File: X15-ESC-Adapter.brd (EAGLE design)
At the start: 101.6 x 41.1 mm, 10 parts, among them J1 IPBT-103-H1-T-S, J2 IPBT-103-H1-T-S, J3 IPBT-103-H1-T-S, J4 IPBT-103-H1-T-S

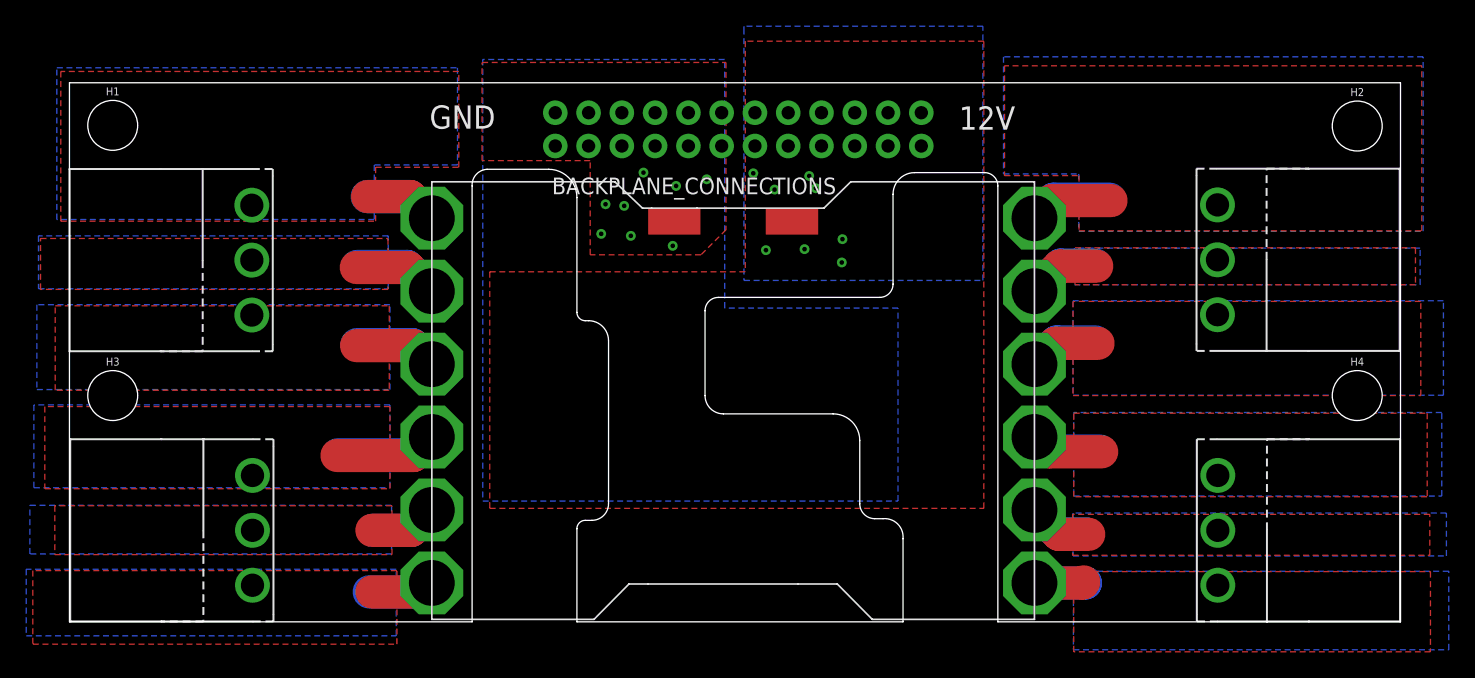
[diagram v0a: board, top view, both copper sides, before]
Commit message: 4th Final Version
Fixed errors
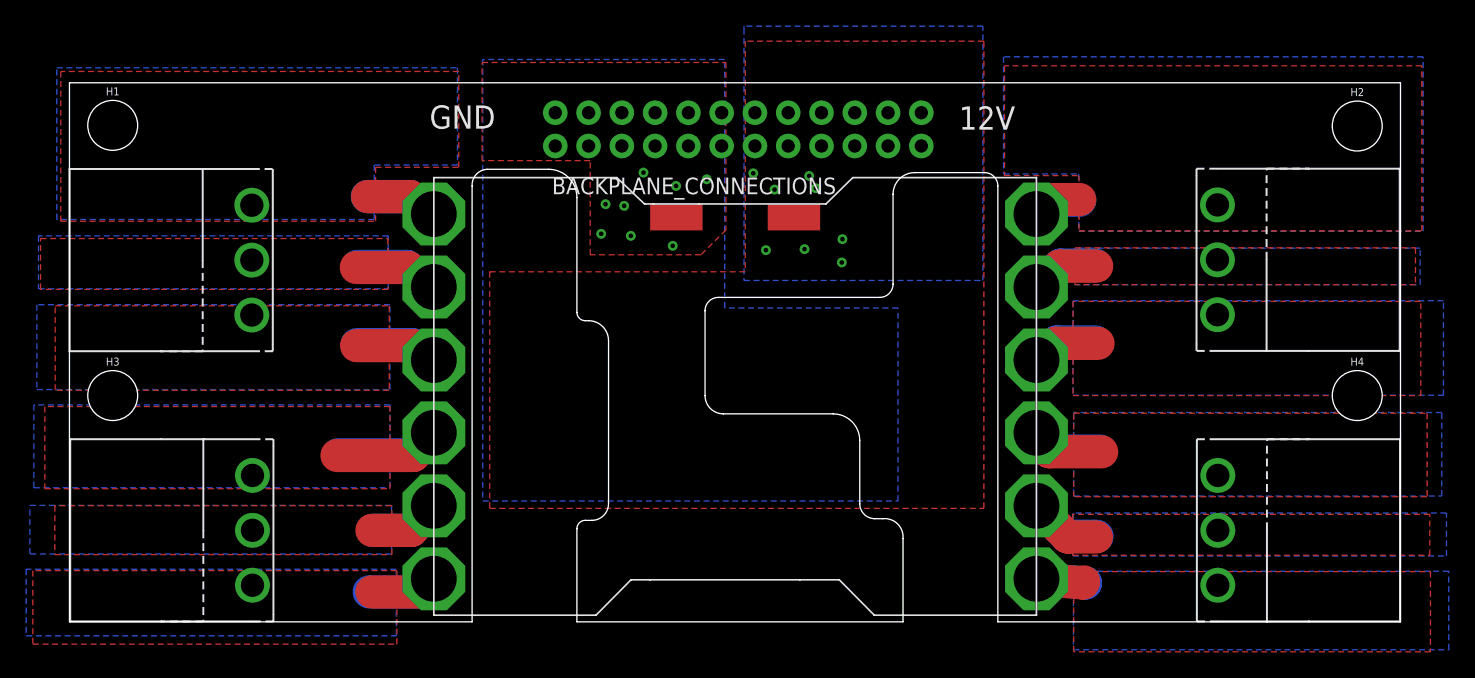
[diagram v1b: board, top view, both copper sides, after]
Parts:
- moved LUMENIER_ESC 0.35 mm to (27.8, 0.51)
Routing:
- net ESC3_B: track 12.7 -> 7.41 mm
- net ESC4_Y: track 9.55 -> 11.1 mm
- net ESC2_R: track 9.91 -> 10.6 mm
- net ESC2_B: track 15.5 -> 16.2 mm
- net ESC2_Y: track 10.4 -> 11.1 mm
- net ESC3_Y: track 11.0 -> 10.4 mm
- net ESC3_R: track 10.9 -> 10.2 mm
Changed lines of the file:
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@@
 <param name="mdViaViaSameLayer" value="6mil"/>
 <param name="mnLayersViaInSmd" value="2"/>
-<param name="mdCopperDimension" value="40mil"/>
+<param name="mdCopperDimension" value="15mil"/>
 <param name="mdDrill" value="6mil"/>
 <param name="mdSmdStop" value="0mil"/>
@@
 <element name="J3" library="X15-ESC-Adapter" package="IPBT-103-H1-T-S" value="IPBT-103-H1-T-S" x="87.63" y="27.6352" smashed="yes" rot="R270"/>
 <element name="J4" library="X15-ESC-Adapter" package="IPBT-103-H1-T-S" value="IPBT-103-H1-T-S" x="87.6554" y="6.985" smashed="yes" rot="R270"/>
-<element name="LUMENIER_ESC" library="X15-ESC-Adapter" package="LUMENIER" package3d_urn="urn:adsk.eagle:package:24294694/3" value="LUMENIER" x="27.66" y="0.1892" smashed="yes"/>
+<element name="LUMENIER_ESC" library="X15-ESC-Adapter" package="LUMENIER" package3d_urn="urn:adsk.eagle:package:24294694/3" value="LUMENIER" x="27.813" y="0.508" smashed="yes"/>
 </elements>
 <signals>
@@
 <vertex x="104.8766" y="24.511"/>
 </polygon>
-<wire x1="73.66" y1="19.6692" x2="75.2506" y2="21.2598" width="2.54" layer="1"/>
+<wire x1="73.813" y1="19.988" x2="75.2506" y2="21.2598" width="2.54" layer="1"/>
 <wire x1="75.2506" y1="21.2598" x2="78.5114" y2="21.2598" width="2.54" layer="1"/>
-<wire x1="73.66" y1="19.6692" x2="75.3522" y2="21.3614" width="2.54" layer="16"/>
+<wire x1="73.813" y1="19.988" x2="75.3522" y2="21.3614" width="2.54" layer="16"/>
 <wire x1="75.3522" y1="21.3614" x2="78.3082" y2="21.3614" width="2.54" layer="16"/>
 </signal>
@@
 <vertex x="103.0986" y="28.5242"/>
 </polygon>
-<wire x1="73.66" y1="25.2392" x2="75.5734" y2="27.1526" width="2.54" layer="1"/>
+<wire x1="73.813" y1="25.558" x2="75.5734" y2="27.1526" width="2.54" layer="1"/>
 <wire x1="75.5734" y1="27.1526" x2="78.4098" y2="27.1526" width="2.54" layer="1"/>
-<wire x1="73.66" y1="25.2392" x2="75.6496" y2="27.2288" width="2.54" layer="16"/>
+<wire x1="73.813" y1="25.558" x2="75.6496" y2="27.2288" width="2.54" layer="16"/>
 <wire x1="75.6496" y1="27.2288" x2="78.3082" y2="27.2288" width="2.54" layer="16"/>
 </signal>
@@
 <vertex x="103.3272" y="43.1292"/>
 </polygon>
-<wire x1="73.66" y1="30.8092" x2="75.0072" y2="32.1564" width="2.54" layer="1"/>
-<wire x1="75.0072" y1="32.1564" x2="79.502" y2="32.1564" width="2.54" layer="1"/>
-<wire x1="73.66" y1="30.8092" x2="75.1088" y2="32.258" width="2.54" layer="16"/>
-<wire x1="75.1088" y1="32.258" x2="79.4004" y2="32.258" width="2.54" layer="16"/>
+<wire x1="73.813" y1="31.128" x2="75.0834" y2="32.2326" width="2.54" layer="1"/>
+<wire x1="75.0834" y1="32.2326" x2="77.1144" y2="32.2326" width="2.54" layer="1"/>
+<wire x1="73.813" y1="31.128" x2="75.0326" y2="32.1818" width="2.54" layer="16"/>
+<wire x1="75.0326" y1="32.1818" x2="77.1144" y2="32.1818" width="2.54" layer="16"/>
 </signal>
 <signal name="ESC4_R">
@@
 <vertex x="105.283" y="3.8608"/>
 </polygon>
-<wire x1="73.66" y1="2.9692" x2="77.3404" y2="2.9692" width="2.54" layer="1"/>
+<wire x1="73.813" y1="3.288" x2="77.3404" y2="2.9692" width="2.54" layer="1"/>
 <wire x1="77.3404" y1="2.9692" x2="77.4192" y2="3.048" width="2.54" layer="1"/>
-<wire x1="73.66" y1="2.9692" x2="77.5436" y2="2.9692" width="2.54" layer="16"/>
+<wire x1="73.813" y1="3.288" x2="77.5436" y2="2.9692" width="2.54" layer="16"/>
 <wire x1="77.5436" y1="2.9692" x2="77.5462" y2="2.9718" width="2.54" layer="16"/>
 </signal>
@@
 <vertex x="105.1052" y="8.3058"/>
 </polygon>
-<wire x1="73.66" y1="8.5392" x2="75.519" y2="6.6802" width="2.54" layer="1"/>
-<wire x1="75.519" y1="6.6802" x2="77.8002" y2="6.6802" width="2.54" layer="1"/>
-<wire x1="73.66" y1="8.5392" x2="75.4682" y2="6.731" width="2.54" layer="16"/>
-<wire x1="75.4682" y1="6.731" x2="77.5462" y2="6.731" width="2.54" layer="16"/>
+<wire x1="73.813" y1="8.858" x2="76.194" y2="6.477" width="2.54" layer="1"/>
+<wire x1="76.194" y1="6.477" x2="78.3844" y2="6.477" width="2.54" layer="1"/>
+<wire x1="73.813" y1="8.858" x2="76.1432" y2="6.5278" width="2.54" layer="16"/>
+<wire x1="76.1432" y1="6.5278" x2="78.4352" y2="6.5278" width="2.54" layer="16"/>
 </signal>
 <signal name="ESC4_B">
@@
 <vertex x="104.7496" y="15.9766"/>
 </polygon>
-<wire x1="73.66" y1="14.1092" x2="74.7898" y2="12.9794" width="2.54" layer="1"/>
+<wire x1="73.813" y1="14.428" x2="74.7898" y2="12.9794" width="2.54" layer="1"/>
 <wire x1="74.7898" y1="12.9794" x2="78.7908" y2="12.9794" width="2.54" layer="1"/>
-<wire x1="73.66" y1="14.1092" x2="74.739" y2="13.0302" width="2.54" layer="16"/>
+<wire x1="73.813" y1="14.428" x2="74.739" y2="13.0302" width="2.54" layer="16"/>
 <wire x1="74.739" y1="13.0302" x2="78.6638" y2="13.0302" width="2.54" layer="16"/>
 </signal>
@@
 <vertex x="-0.9652" y="30.7086"/>
 </polygon>
-<wire x1="27.66" y1="30.8092" x2="26.008" y2="32.4612" width="2.54" layer="1"/>
+<wire x1="27.813" y1="31.128" x2="26.008" y2="32.4612" width="2.54" layer="1"/>
 <wire x1="26.008" y1="32.4612" x2="22.7584" y2="32.4612" width="2.54" layer="1"/>
-<wire x1="27.66" y1="30.8092" x2="26.008" y2="32.4612" width="2.54" layer="16"/>
+<wire x1="27.813" y1="31.128" x2="26.008" y2="32.4612" width="2.54" layer="16"/>
 <wire x1="26.008" y1="32.4612" x2="22.733" y2="32.4612" width="2.54" layer="16"/>
 </signal>
@@
 <vertex x="24.9936" y="3.9116"/>
 </polygon>
-<wire x1="27.66" y1="2.9692" x2="26.9768" y2="2.286" width="2.54" layer="1"/>
+<wire x1="27.813" y1="3.288" x2="26.9768" y2="2.286" width="2.54" layer="1"/>
 <wire x1="26.9768" y1="2.286" x2="23.0886" y2="2.286" width="2.54" layer="1"/>
-<wire x1="27.66" y1="2.9692" x2="26.9768" y2="2.286" width="2.54" layer="16"/>
+<wire x1="27.813" y1="3.288" x2="26.9768" y2="2.286" width="2.54" layer="16"/>
 <wire x1="26.9768" y1="2.286" x2="22.8854" y2="2.286" width="2.54" layer="16"/>
 </signal>
@@
 <vertex x="-3.0226" y="8.89"/>
 </polygon>
-<wire x1="27.66" y1="8.5392" x2="26.1058" y2="6.985" width="2.54" layer="1"/>
+<wire x1="27.813" y1="8.858" x2="26.1058" y2="6.985" width="2.54" layer="1"/>
 <wire x1="26.1058" y1="6.985" x2="23.0886" y2="6.985" width="2.54" layer="1"/>
-<wire x1="27.66" y1="8.5392" x2="26.1058" y2="6.985" width="2.54" layer="16"/>
+<wire x1="27.813" y1="8.858" x2="26.1058" y2="6.985" width="2.54" layer="16"/>
 <wire x1="26.1058" y1="6.985" x2="23.1394" y2="6.985" width="2.54" layer="16"/>
 </signal>
@@
 <vertex x="24.4602" y="16.5608"/>
 </polygon>
-<wire x1="27.66" y1="14.1092" x2="26.2508" y2="12.7" width="2.54" layer="1"/>
+<wire x1="27.813" y1="14.428" x2="26.2508" y2="12.7" width="2.54" layer="1"/>
 <wire x1="26.2508" y1="12.7" x2="20.4216" y2="12.7" width="2.54" layer="1"/>
-<wire x1="27.66" y1="14.1092" x2="26.3016" y2="12.7508" width="2.54" layer="16"/>
+<wire x1="27.813" y1="14.428" x2="26.3016" y2="12.7508" width="2.54" layer="16"/>
 <wire x1="26.3016" y1="12.7508" x2="20.4978" y2="12.7508" width="2.54" layer="16"/>
 </signal>
@@
 <vertex x="24.4602" y="24.2062"/>
 </polygon>
-<wire x1="27.66" y1="19.6692" x2="26.2472" y2="21.082" width="2.54" layer="1"/>
+<wire x1="27.813" y1="19.988" x2="26.2472" y2="21.082" width="2.54" layer="1"/>
 <wire x1="26.2472" y1="21.082" x2="21.9202" y2="21.082" width="2.54" layer="1"/>
-<wire x1="27.66" y1="19.6692" x2="26.171" y2="21.1582" width="2.54" layer="16"/>
+<wire x1="27.813" y1="19.988" x2="26.171" y2="21.1582" width="2.54" layer="16"/>
 <wire x1="26.171" y1="21.1582" x2="21.9456" y2="21.1582" width="2.54" layer="16"/>
 </signal>
@@
 <vertex x="24.3332" y="29.464"/>
 </polygon>
-<wire x1="27.66" y1="25.2392" x2="25.8482" y2="27.051" width="2.54" layer="1"/>
+<wire x1="27.813" y1="25.558" x2="25.8482" y2="27.051" width="2.54" layer="1"/>
 <wire x1="25.8482" y1="27.051" x2="21.8948" y2="27.051" width="2.54" layer="1"/>
-<wire x1="27.66" y1="25.2392" x2="25.772" y2="27.1272" width="2.54" layer="16"/>
+<wire x1="27.813" y1="25.558" x2="25.772" y2="27.1272" width="2.54" layer="16"/>
 <wire x1="25.772" y1="27.1272" x2="21.971" y2="27.1272" width="2.54" layer="16"/>
 </signal>
@@
 <mfgpreviewcolor name="substratecolor" color="0xFF786E46"/>
 </mfgpreviewcolors>
-<errors>
-</errors>
 </board>
 </drawing>
